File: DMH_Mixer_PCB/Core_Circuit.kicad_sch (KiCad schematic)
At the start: 42 parts, among them SW1 SW_SPDT_321, SW2 SW_SPDT_321, SW3 SW_SPDT_321, SW4 SW_SPDT_321, U1 TL074

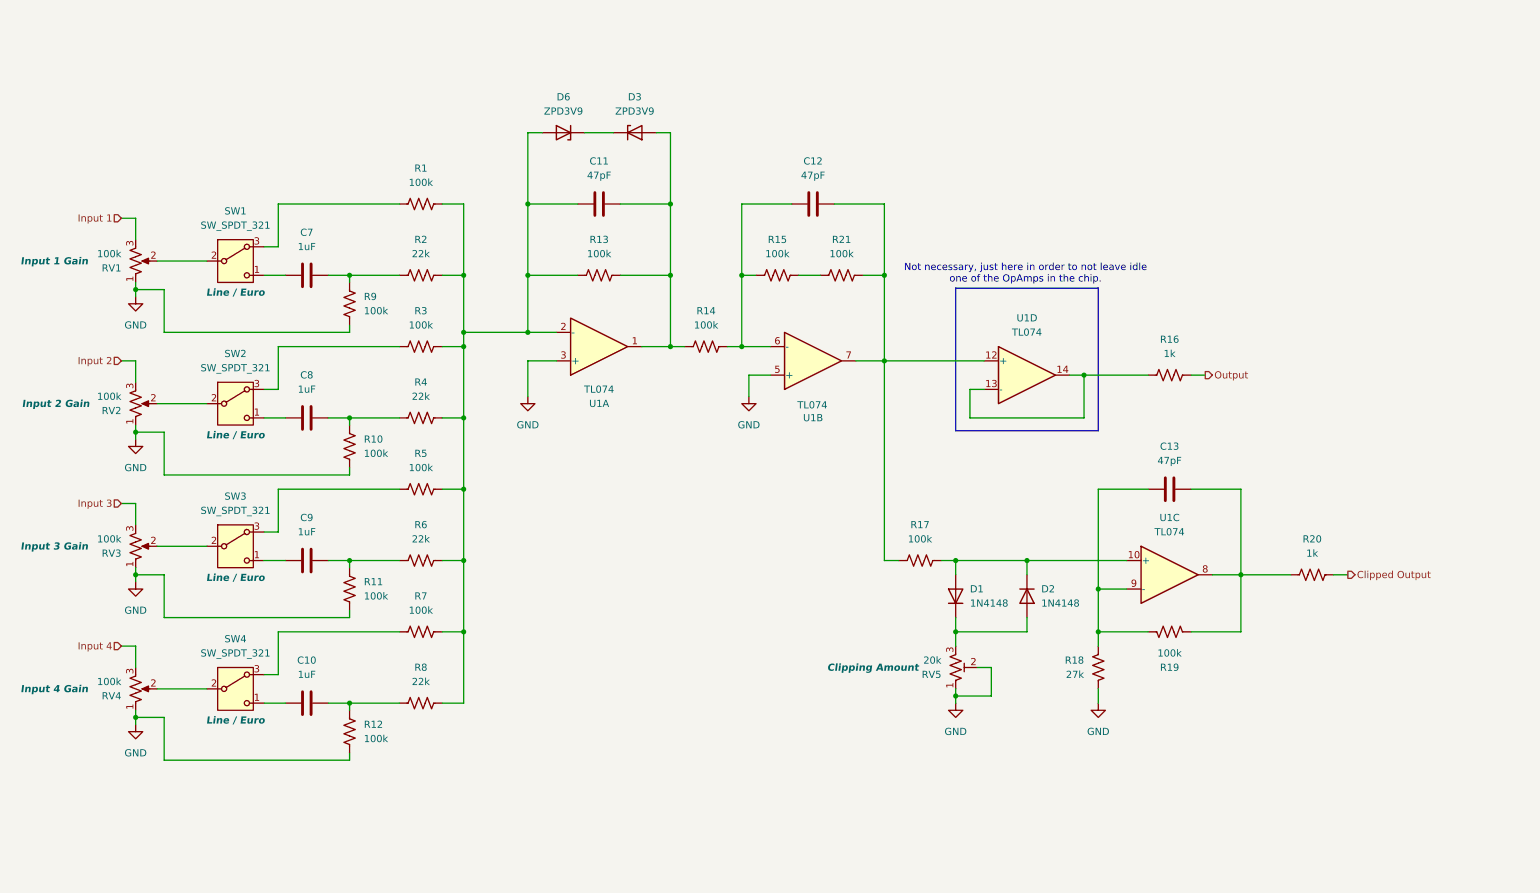
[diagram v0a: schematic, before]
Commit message: Output selection in progress
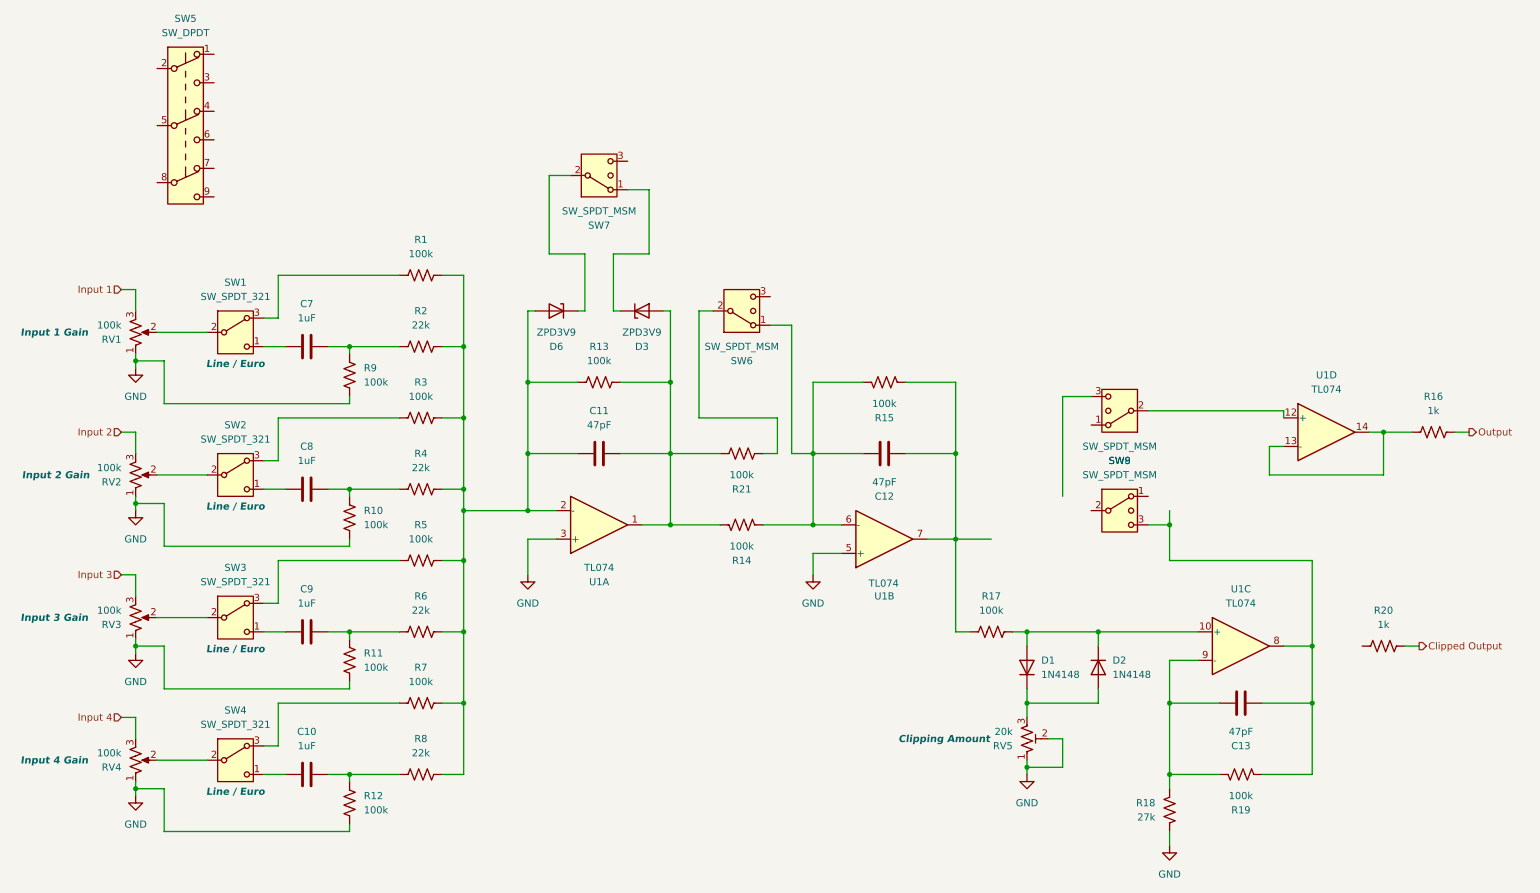
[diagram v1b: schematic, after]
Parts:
- added SW5: SW_DPDT, SynthStuff:PinHeader_2x03_P2.54mm_Vertical_142536, symbol SynthStuff:Switch_3PDT
- added SW6, SW7, SW8, SW9: SW_SPDT_MSM, symbol Switch:SW_SPDT_MSM
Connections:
- net at C13.2, R19.2, U1.8: now also SW9.3 (4); no longer R20.1
- net at C12.2, R17.1, U1.7: now also R15.2; no longer R21.2, U1.12 (+)
- net at D3.1 (K): now also SW7.1; no longer D6.1 (K)
- net at C11.2, D3.2 (A), R13.2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: now also R21.2
- net at R21.1: now also SW6.2 (3); no longer R15.2
- net at C12.1, R14.2, R15.1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: now also SW6.1
- new net: SW8.2 (3), U1.12 (+)
- new net: D6.1 (K), SW7.2 (3)
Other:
- note removed: "Not necessary, just here in order to not leave idle one of the OpAmps in the chip."
- moved on the sheet: C10, C11, C12, C13, C7, C8, C9, D1, D2, D3, D6, R1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
